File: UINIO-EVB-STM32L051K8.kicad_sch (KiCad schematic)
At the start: 19 parts

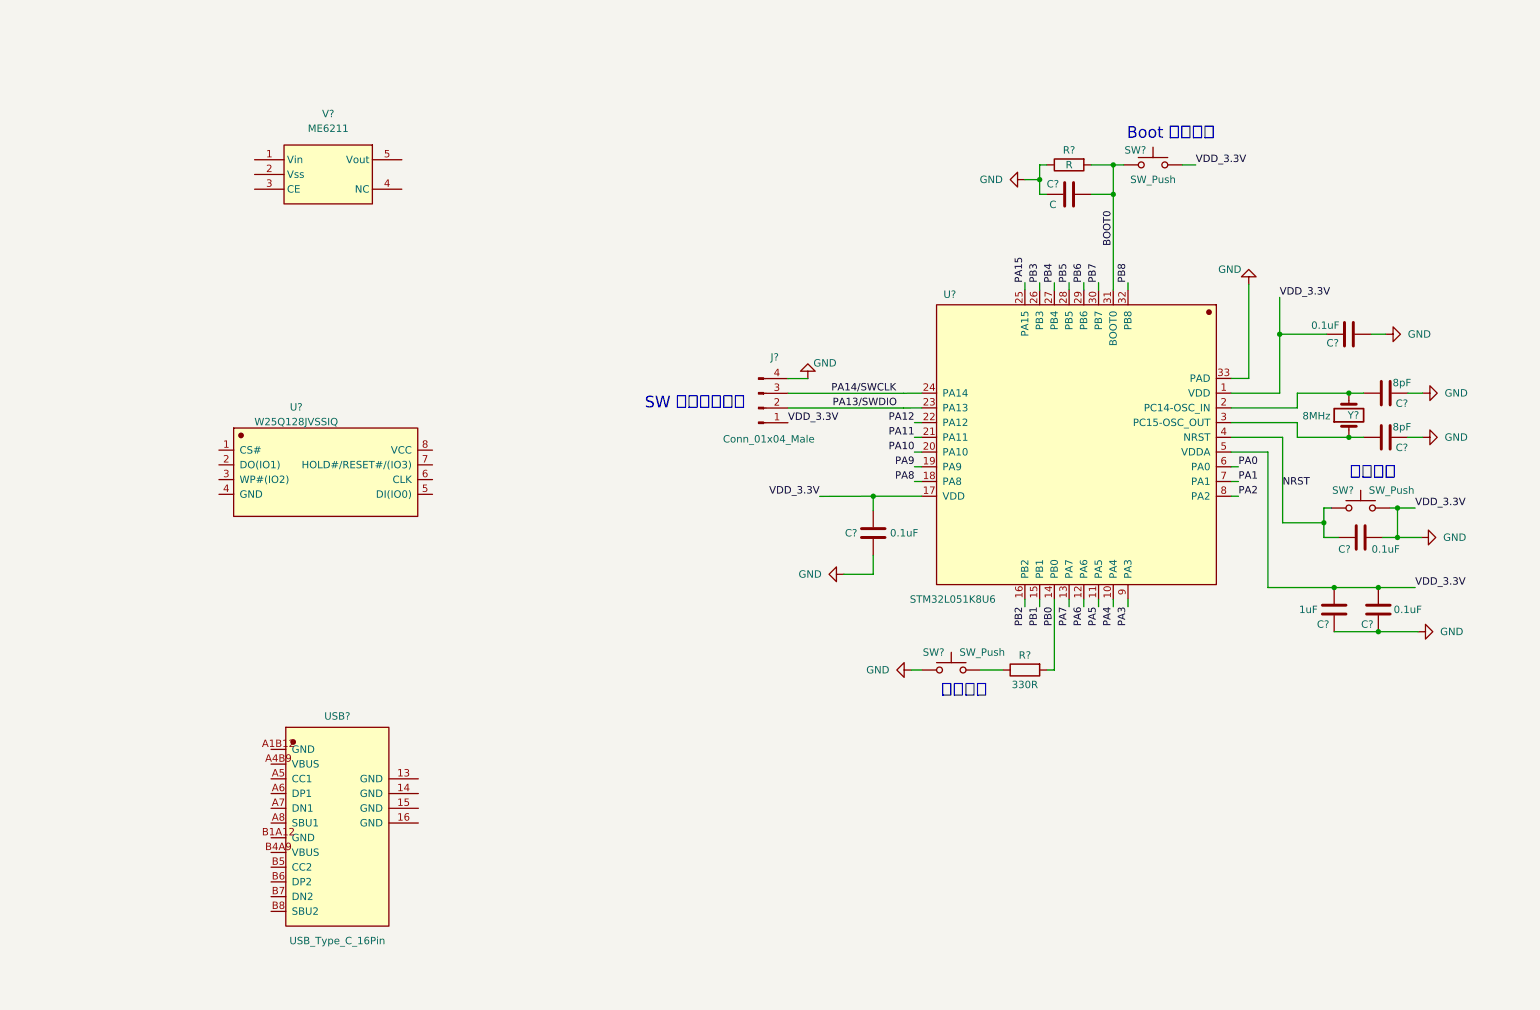
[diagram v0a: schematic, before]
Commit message: update
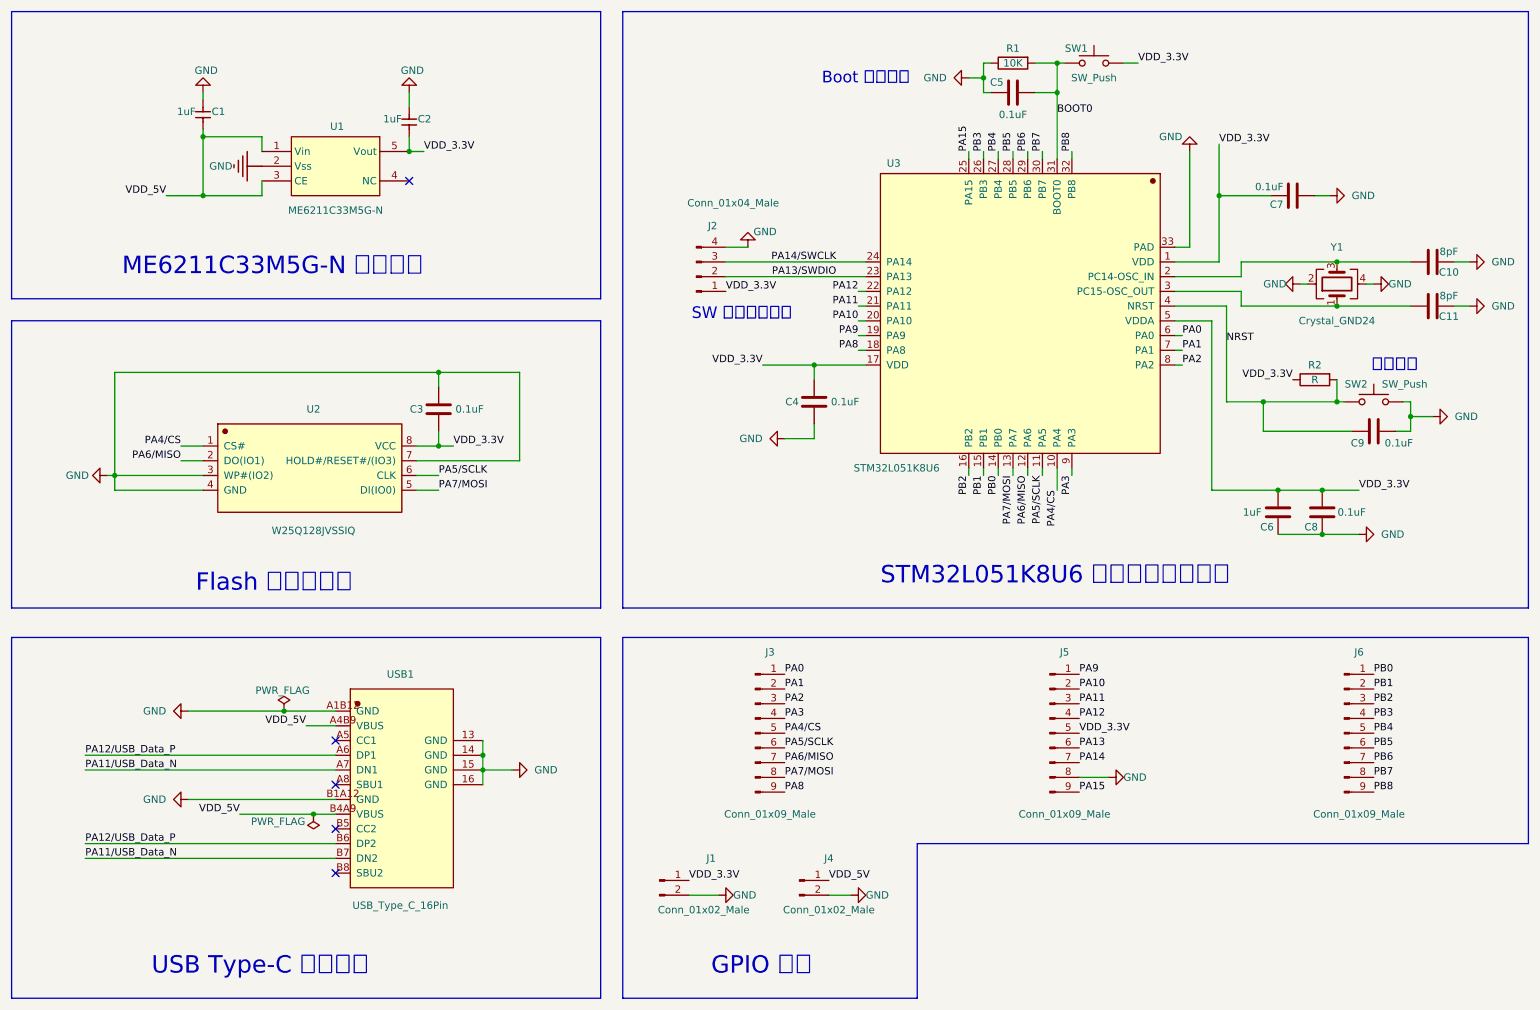
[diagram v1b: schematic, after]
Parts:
- removed R?: 330R, symbol Device:R
- removed SW?: SW_Push, symbol Switch:SW_Push
- removed USB?: USB_Type_C_16Pin, Uinio:USB-C-SMD_TYPEC-304J-BCP16, symbol Uinio:USB_Type_C_16Pin
- removed V?: ME6211, Uinio:SOT23-5, symbol Uinio:ME6211
- removed Y?: 8MHz, symbol Device:Crystal
- added C1, C2: 1uF, Capacitor_SMD:C_0603_1608Metric, symbol Uinio:CAP_0402
- added C3: 0.1uF, symbol Device:C
- added J1, J4: Conn_01x02_Male, symbol Connector:Conn_01x02_Male
- added J3, J5, J6: Conn_01x09_Male, symbol Connector:Conn_01x09_Male
- added R2: R, symbol Device:R
- added U1: ME6211C33M5G-N, Uinio:SOT-23-5_L3.0-W1.7-P0.95-LS2.8-BR, symbol Uinio:ME6211
- added USB1: USB_Type_C_16Pin, Uinio:USB-C-SMD_TYPEC-304J-BCP16, symbol Uinio:USB_Type_C_16Pin
- added Y1: Crystal_GND24, symbol Device:Crystal_GND24
- C5: renamed from C?; value C -> 0.1uF
- R1: renamed from R?; value R -> 10K
- gave numbers to parts that had none: 12
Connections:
- net PA4 is gone; now on net PA4/CS: U3.10 (PA4)
- net PA5 is gone; now on net PA5/SCLK: U3.11 (PA5)
- net PA6 is gone; now on net PA6/MISO: U3.12 (PA6)
- net PA7 is gone; now on net PA7/MOSI: U3.13 (PA7)
- net GND: now also U2.3 (WP#(IO2)), U2.4 (GND), U2.7 (HOLD#/RESET#/(IO3)), C1.1, C2.1, C3.1, J1.2 (Pin_2), J4.2 (Pin_2), J5.8 (Pin_8), U1.2 (Vss), USB1.13 (GND), USB1.14 (GND), USB1.15 (GND), USB1.16 (GND), USB1.A1B12 (GND), USB1.B1A12 (GND), Y1.2, Y1.4; no longer C4.1, C6.2, C7.2, C8.2, J2.1 (Pin_1), SW1.1, U3.1 (VDD), U3.17 (VDD), U3.5 (VDDA)
- net NRST: now also R2.2
- net PA0: now also J3.1 (Pin_1)
- net PA1: now also J3.2 (Pin_2)
- net PA10: now also J5.2 (Pin_2)
- net PA11: now also J5.3 (Pin_3)
- net PA12: now also J5.4 (Pin_4)
- net PA15: now also J5.9 (Pin_9)
- net PA2: now also J3.3 (Pin_3)
- net PA3: now also J3.4 (Pin_4)
- net PA8: now also J3.9 (Pin_9)
- net PA9: now also J5.1 (Pin_1)
- net PB0: now also J6.1 (Pin_1)
- net PB1: now also J6.2 (Pin_2)
- net PB2: now also J6.3 (Pin_3)
- net PB3: now also J6.4 (Pin_4)
- net PB4: now also J6.5 (Pin_5)
- net PB5: now also J6.6 (Pin_6)
- net PB6: now also J6.7 (Pin_7)
- net PB7: now also J6.8 (Pin_8)
- net PB8: now also J6.9 (Pin_9)
- net at C10.2, U3.2 (PC14-OSC_IN): now also Y1.3
- net at C11.2, U3.3 (PC15-OSC_OUT): now also Y1.1
- net PA4/CS: now reaches U2.1 (CS#)
- net PA4/CS: now also J3.5 (Pin_5)
- net PA6/MISO: now reaches U2.2 (DO(IO1))
- net PA6/MISO: now also J3.7 (Pin_7)
- net PA7/MOSI: now reaches U2.5 (DI(IO0))
- net PA7/MOSI: now also J3.8 (Pin_8)
- net PA5/SCLK: now reaches U2.6 (CLK)
- net PA5/SCLK: now also J3.6 (Pin_6)
- net VDD_3.3V: now reaches U2.8 (VCC)
- net VDD_3.3V: now also C4.1, C6.2, C7.2, C8.2, J2.1 (Pin_1), SW1.1, U3.1 (VDD), U3.17 (VDD), U3.5 (VDDA), C2.2, C3.2, J1.1 (Pin_1), J5.5 (Pin_5), R2.1, U1.5 (Vout)
- new net PA11/USB_Data_N: USB1.A7 (DN1), USB1.B7 (DN2)
- new net PA12/USB_Data_P: USB1.A6 (DP1), USB1.B6 (DP2)
- new net PA13: J5.6 (Pin_6)
- new net PA14: J5.7 (Pin_7)
- new net VDD_5V: C1.2, J4.1 (Pin_1), U1.1 (Vin), U1.3 (CE), USB1.A4B9 (VBUS), USB1.B4A9 (VBUS)
- no-connect marks 0 -> 5
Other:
- note added: "Flash 存储器电路"
- note added: "GPIO 插座"
- note added: "ME6211C33M5G-N 供电电路"
- note added: "STM32L051K8U6 微控制器最小系统"
- note added: "USB Type-C 接口电路"
- note removed: "用户按键"
- company: (none) -> UinIO.com
- title: (none) -> UINIO-EVB-STM32L051K8
- moved on the sheet: C10, C11, C4, C5, C6, C7, C8, C9, J2, R1, SW1, SW2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

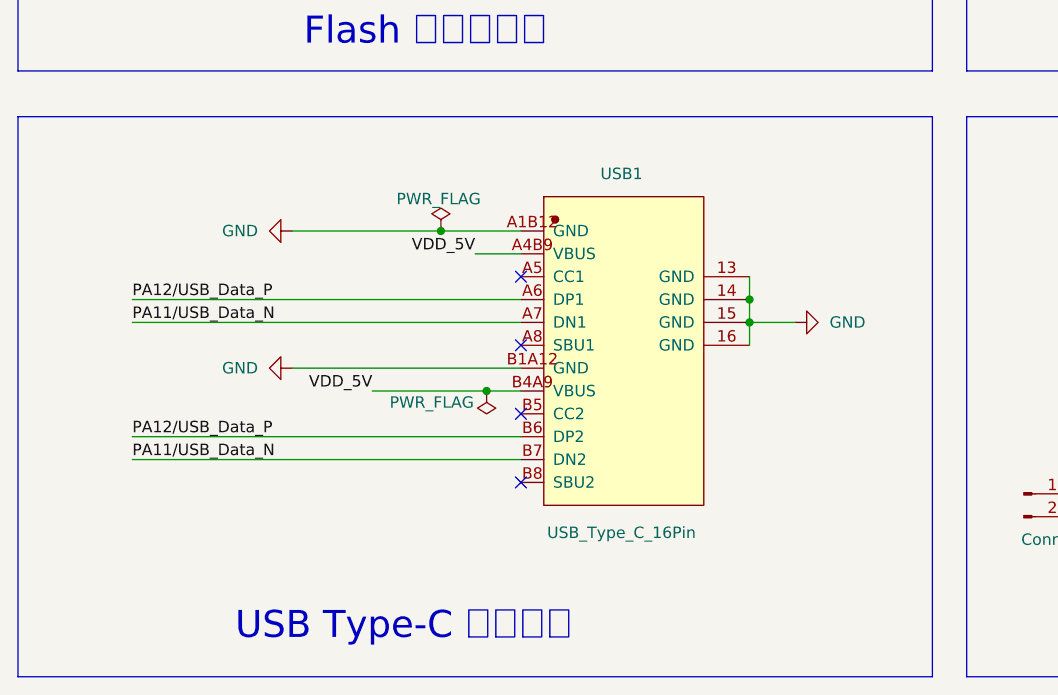
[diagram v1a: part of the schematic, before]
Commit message: Schematic is complete.
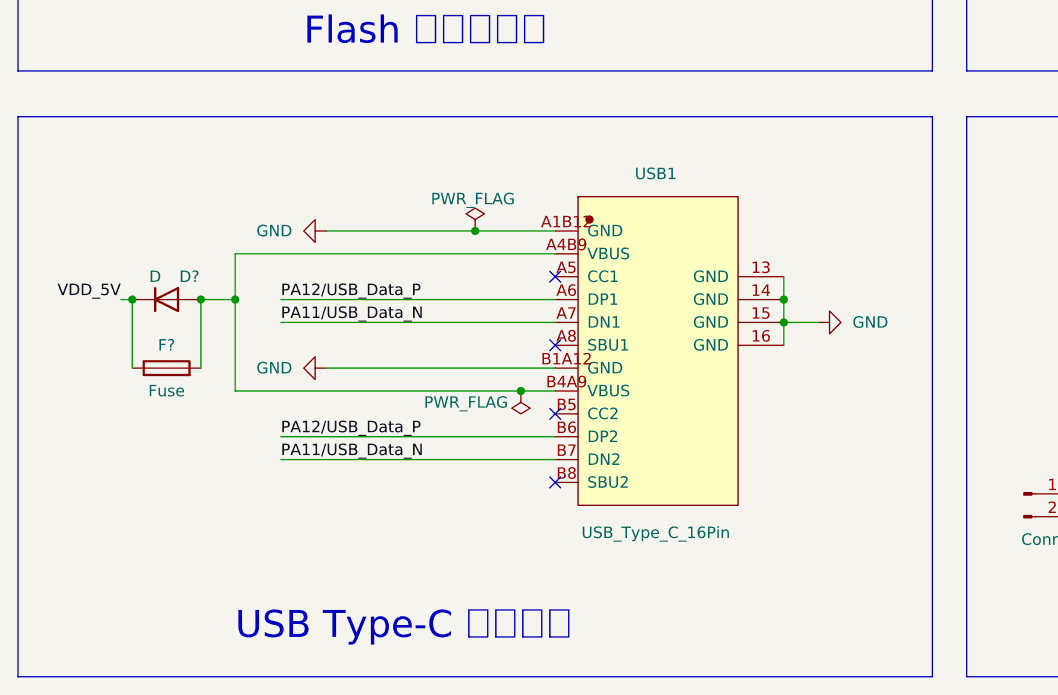
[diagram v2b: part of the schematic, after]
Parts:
- added D?: D, symbol Device:D
- added F?: Fuse, symbol Device:Fuse
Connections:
- net VDD_5V: now also D?.1 (K), F?.1; no longer USB1.A4B9 (VBUS), USB1.B4A9 (VBUS)
- new net: D?.2 (A), F?.2, USB1.A4B9 (VBUS), USB1.B4A9 (VBUS)
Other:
- moved on the sheet: USB1
